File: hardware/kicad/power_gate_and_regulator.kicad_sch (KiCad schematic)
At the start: 13 parts, among them Q2 DMG3415U-7, Q2 PMV32UP, U4 XC6220, U5 TPL5110

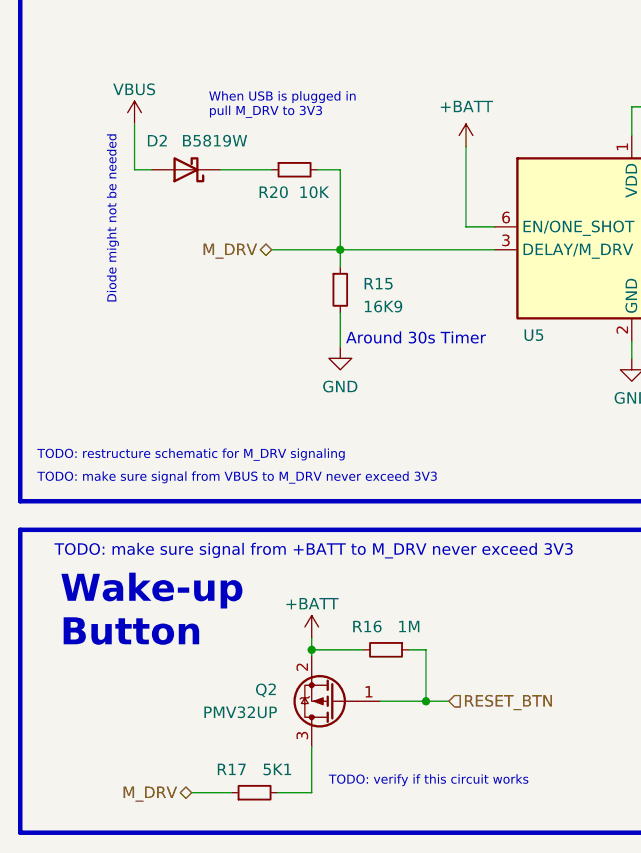
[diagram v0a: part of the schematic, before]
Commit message: wip wake up button
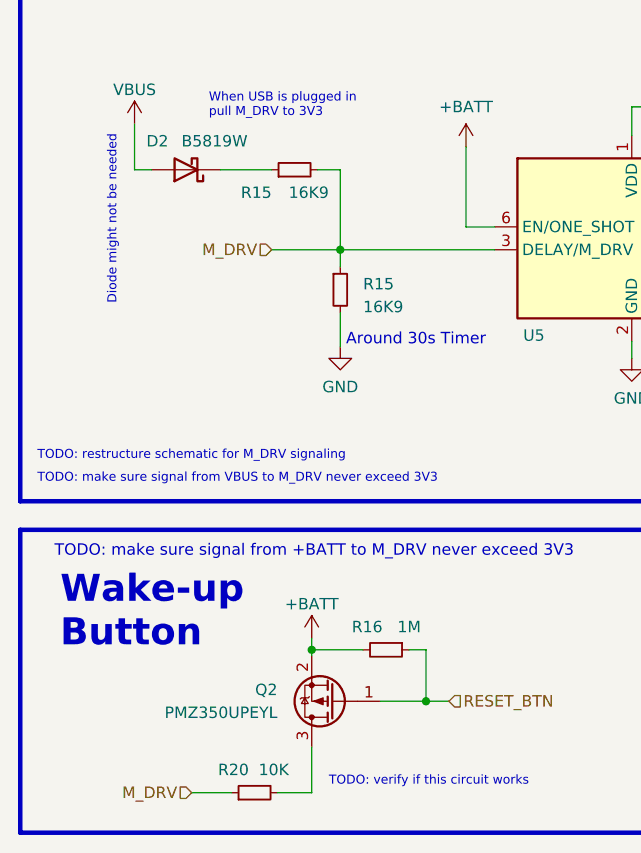
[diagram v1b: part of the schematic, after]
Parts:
- removed R17: 5K1, Resistor_SMD:R_0402_1005Metric, symbol Device:R_Small
- added R15: 16K9, Resistor_SMD:R_0402_1005Metric, symbol Device:R_Small
- Q2: value PMV32UP -> PMZ350UPEYL; footprint Package_TO_SOT_SMD:SOT-23 -> Package_TO_SOT_SMD:SOT-883; Distributor Link https://www.lcsc.com/product-detail/MOSFETs_TECH-PUBLIC-PMV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 -> https://www.lcsc.com/product-detail/MOSFETs_Nexperia-PMZ350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; Distributor Part Number C2959851 -> C478207; Manufacturer TECH PUBLIC -> Nexperia; Manufacturer Part Number PMV32UP -> PMZ350UPEYL; Part Description MOSFET P Channel 20V 4A 52mΩ@4.5V -> MOSFET P Channel 20V 1A 450mΩ@4.5V,300mA 360mW
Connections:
- net M_DRV: now also R20.1, R15.2; no longer R20.2
- net at D2.1 (K): now also R15.1; no longer R20.1
- net at Q2.3 (D): now also R20.2
